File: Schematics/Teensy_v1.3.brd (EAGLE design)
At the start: 84.8 x 65.4 mm, 43 parts, among them IC5 SN, IC6 YM, IC7 7.68MHz, IC8 3.57MHz, J1 OLED_128X64_I2C, J3 POWER_JACK

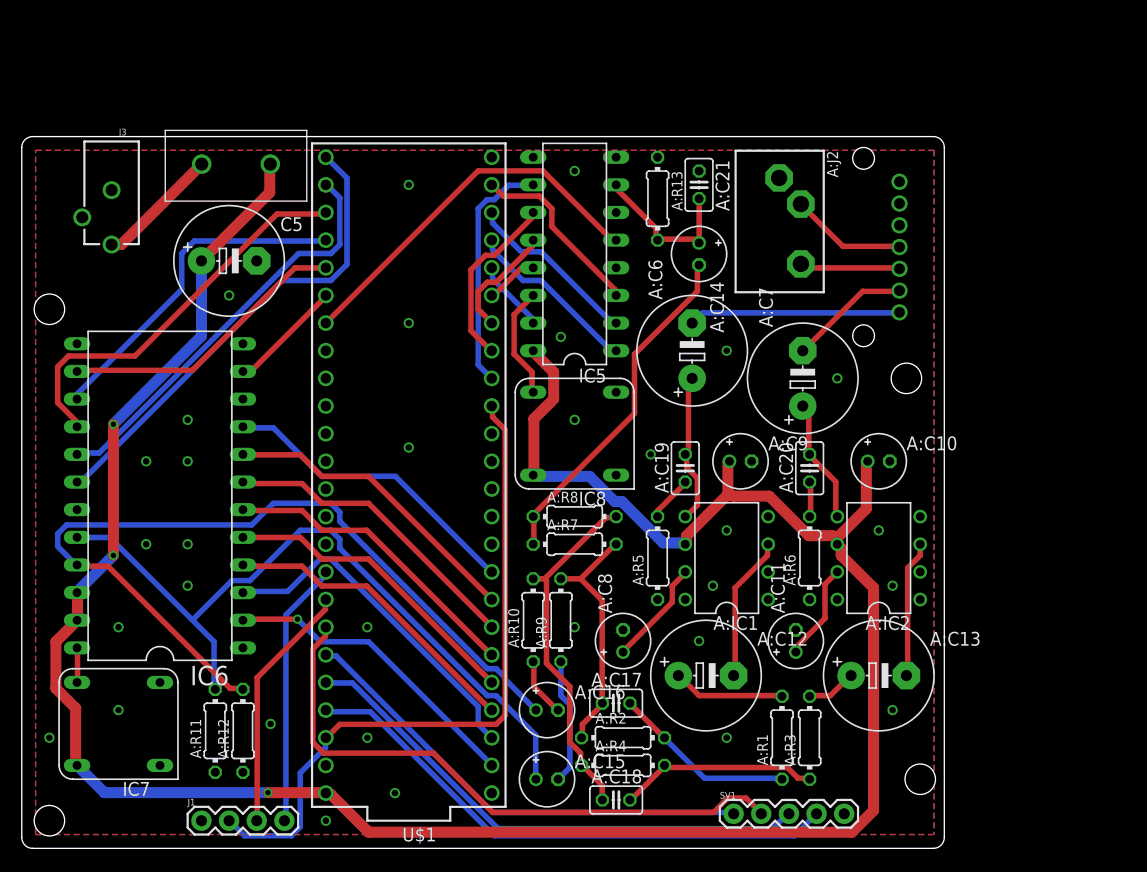
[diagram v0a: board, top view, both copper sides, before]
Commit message: Total Resdesign
This should probably be considered a 2.0 rev
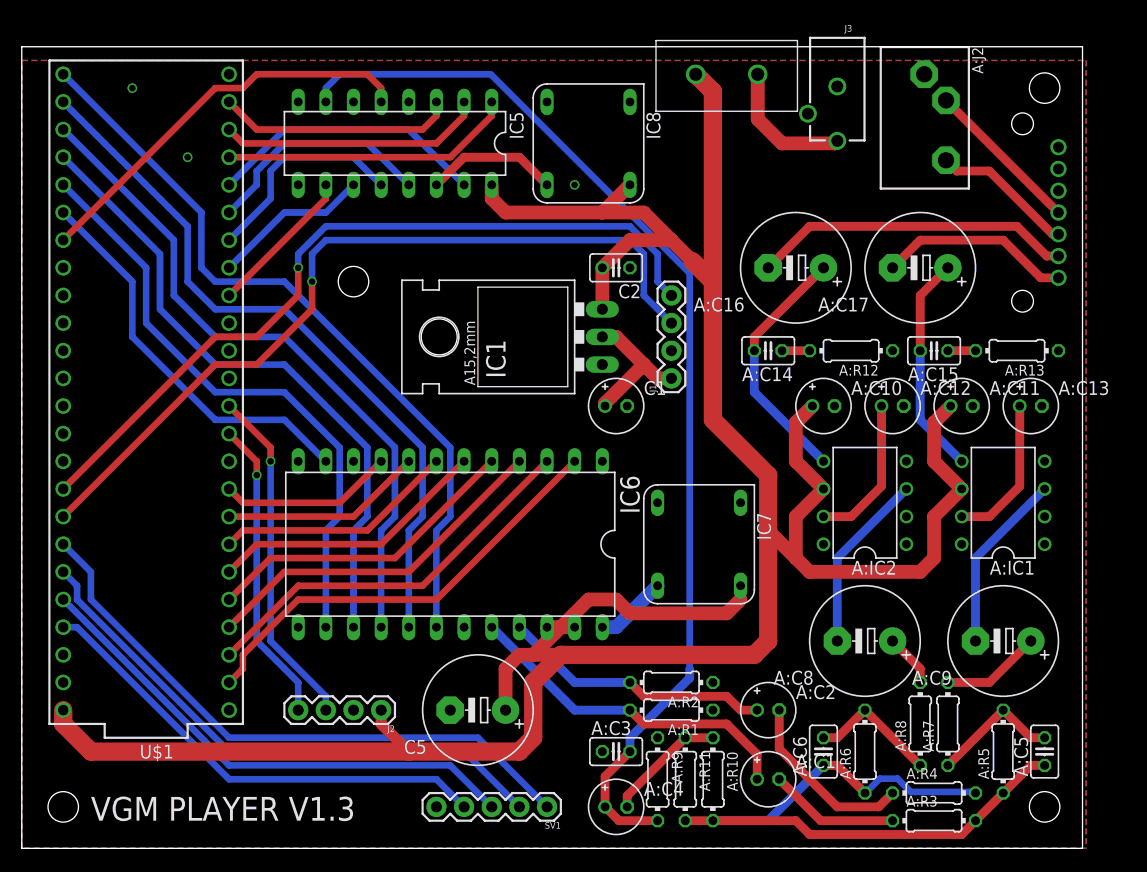
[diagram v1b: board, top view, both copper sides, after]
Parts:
- removed A:C18: 4.7nF, resistor:C025-025X050
- removed A:C19, A:C20: 47nF, resistor:C025-025X050
- removed A:C21: 220pF, resistor:C025-025X050
- removed A:C7: 1000uF, resistor:E5-10,5
- added A:C1, A:C2, C1: 10uF, resistor:E2-5
- added A:C3: 220pF, resistor:C025-025X050
- added A:C4: 1uF, resistor:E2-5
- added A:C5: 4.7nF, resistor:C025-025X050
- added C2: 100nF, resistor:C025-025X050
- added IC1: LD117AV33, v-reg:TO220L1
- added J2: HC-06, SparkFun-Connectors:1X04
- A:C12, A:C13: value 16uF -> 100uF; device resistor:E5-10,5 -> resistor:E2-5
- A:C14: value 1uF -> 47nF; device resistor:E2-5 -> resistor:C025-025X050
- A:C15: value 10uF -> 47nF; device resistor:E2-5 -> resistor:C025-025X050
- A:C16: value 10uF -> 1000uF; device resistor:E2-5 -> resistor:E5-10,5
- A:C17: value 4.7nF -> 1000uF; device resistor:C025-025X050 -> resistor:E5-10,5
- A:C6: value 1000uF -> 4.7nF; device resistor:E5-10,5 -> resistor:C025-025X050
- A:C8, A:C9: value 100uF -> 16uF; device resistor:E2-5 -> resistor:E5-10,5
- A:R1, A:R3: value 11k -> 2.2k
- A:R10, A:R11: value 2.2k -> 51k
- A:R12, A:R13: value 2.2k -> 10
- A:R2, A:R4: value 10k -> 2.2k
- A:R5, A:R6: value 10 -> 10k
- A:R7, A:R8: value 51k -> 11k
- moved J3 67.4 mm to (74.9, 76.2)
- moved A:R12 65.9 mm to (76.2, 45.7), turned to 180 degrees
- moved J1 59.3 mm to (59.7, 43.2), turned to 90 degrees
- moved IC7 55.8 mm to (62.2, 27.9), turned to 180 degrees
- moved A:C15 53.1 mm to (83.8, 45.7), turned to 180 degrees
- moved A:C17 48.8 mm to (82.5, 53.3), turned to 180 degrees
- moved C5 47.2 mm to (41.9, 12.7), turned to 180 degrees
- moved A:C16 46.6 mm to (71.1, 53.3), turned to 180 degrees
- moved U$7 45.8 mm to (64.8, 71.1)
- moved A:R11 43.4 mm to (61.0, 6.35), turned to 270 degrees
- moved A:C6 38.8 mm to (73.7, 8.89)
- moved A:R7 38.1 mm to (85.1, 11.4), turned to 90 degrees
- moved A:R8 37.0 mm to (82.5, 11.4), turned to 90 degrees
- moved A:R5 36.4 mm to (90.2, 8.89)
- moved A:R13 35.9 mm to (91.4, 45.7), turned to 180 degrees
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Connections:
- net NEXT_BUTTON renamed BUTTON4
- net RAND_BUTTON renamed BUTTON3
- removed net 3V3: J1.1, U$1.3.3V, U$1.3.3V3
- removed net N$2: J3.PWR, U$7.P$1
- removed net PAUSE: SV1.2, U$1.20/A6
- removed net PREV_BUTTON: SV1.1, U$1.21/A7
- new net 3.3V: U$1.3.3V
- new net BUTTON1: SV1.1, U$1.20/A6
- new net BUTTON2: SV1.2, U$1.21/A7
- new net N$3: J3.PWR, U$7.P$2
- new net RX: J2.3, U$1.10
- new net TX: J2.4, U$1.9
- new net VCC: C1.+, IC1.2, J1.1
- net 5V: now also A:C11.+, C2.2, IC1.3, J2.1, U$7.P$1; no longer A:C9.+, U$7.P$2
- net A:N$1: now also A:C16.-; no longer A:C7.-
- net A:N$10: now also A:C8.+, A:R8.2; no longer A:C13.+, A:R3.2
- net A:N$11: now also A:C15.1, A:R13.2; no longer A:C19.1, A:R5.2
- net A:N$12: now also A:C14.1, A:R12.2; no longer A:C20.1, A:R6.2
- net A:N$13: now also A:C6.1, A:R4.2, A:R6.1; no longer A:C18.1, A:R4.1, A:R8.2
- net A:N$14: now also A:C5.1, A:R11.2, A:R3.2, A:R5.1; no longer A:C17.1, A:R2.1, A:R7.2, A:R9.2
- net A:N$15: now also A:C4.-, A:R10.1, A:R11.1; no longer A:C14.-, A:R7.1, A:R8.1
- net A:N$16: now also A:C1.-, A:R3.1; no longer A:C15.-, A:R9.1
- net A:N$17: now also A:C2.-, A:R4.1; no longer A:C16.-, A:R10.1
- net A:N$18: now also A:C5.2, A:R5.2, A:R7.1; no longer A:C17.2, A:R1.1, A:R2.2
- net A:N$19: now also A:C6.2, A:R6.2, A:R8.1; no longer A:C18.2, A:R3.1, A:R4.2
- net A:N$2: now also A:C17.-; no longer A:C6.-
- net A:N$3: now also A:C15.2, A:C17.+; no longer A:C19.2, A:C6.+
- net A:N$4: now also A:C14.2, A:C16.+; no longer A:C20.2, A:C7.+
- net A:N$5: now also A:C13.+; no longer A:C8.+
- net A:N$6: now also A:C12.+; no longer A:C11.+
- net A:N$7: now also A:C9.-; no longer A:C12.-
- net A:N$8: now also A:C8.-; no longer A:C13.-
- net A:N$9: now also A:C9.+, A:R7.2; no longer A:C12.+, A:R1.2
- net GND: now also A:C12.-, A:C13.-, A:C3.1, A:R1.1, A:R2.1, A:R9.1, C1.-, C2.1, IC1.1, J2.2, J3.GNDBREAK; no longer A:C21.1, A:C8.-, A:C9.-, A:R11.1, A:R5.1, A:R6.1
- net SN_OUT: now also A:C3.2, A:C4.+, A:R9.2; no longer A:C14.+, A:C21.2, A:R13.2
- net YM_MOL: now also A:C2.+, A:R2.2; no longer A:C16.+, A:R12.2
- net YM_MOR: now also A:C1.+, A:R1.2; no longer A:C15.+, A:R11.2
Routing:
- net SN_OUT: track 14.8 -> 100.4 mm
- net 3V3: track 62.7 -> 0.00 mm
- net PAUSE: track 56.1 -> 0.00 mm
- net BUTTON1: track 0.00 -> 55.9 mm
- net YM_MOL: track 77.2 -> 25.0 mm
- net I2C_SCL: track 22.9 -> 74.8 mm, vias 0 -> 1
- net BUTTON2: track 0.00 -> 51.6 mm
- net I2C_SDA: track 24.4 -> 72.2 mm, vias 0 -> 1
- net PREV_BUTTON: track 43.6 -> 0.00 mm
- net YM_MOR: track 68.3 -> 31.5 mm
- net 5V: track 225.9 -> 258.4 mm, vias 3 -> 0
- net RX: track 0.00 -> 31.6 mm, vias 0 -> 1
- net YM_CS: track 26.8 -> 55.4 mm
- net TX: track 0.00 -> 28.0 mm, vias 0 -> 1
- net YM_A0: track 38.2 -> 66.2 mm
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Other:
- board size 84.8 x 65.4 mm -> 97.5 x 73.7 mm
- board text added: "VGM PLAYER V1.3"
